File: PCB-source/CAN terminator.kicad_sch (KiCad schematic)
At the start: 6 parts, among them U8 TLP175A, U9 TLP175A

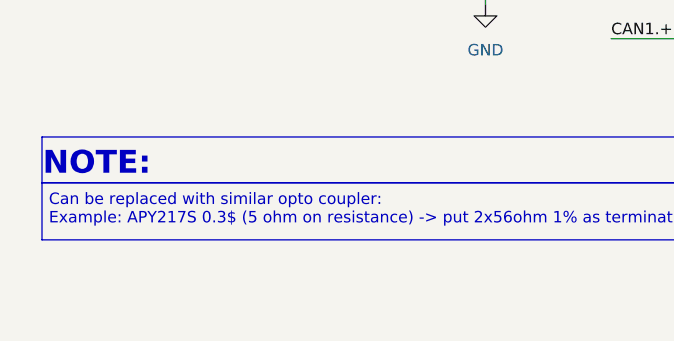
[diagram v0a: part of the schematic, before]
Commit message: bom done
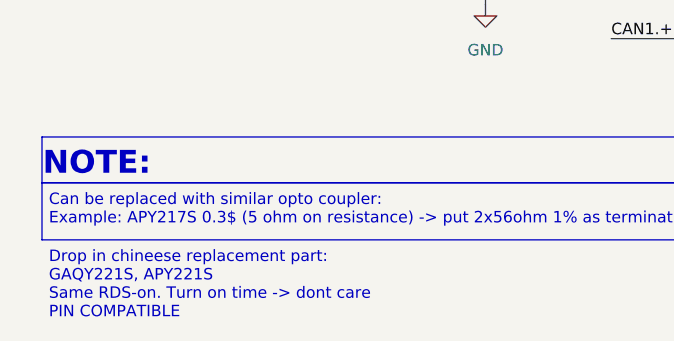
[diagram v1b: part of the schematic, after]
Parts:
- U8, U9: LCSC (none) -> C141522
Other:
- note added: "Drop in chineese replacement part: GAQY221S, APY221S Same RDS-on. Turn on time -> dont care PIN COMPATIBLE"
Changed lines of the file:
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@@
+		)
+	)
+	(text "Drop in chineese replacement part:\nGAQY221S, APY221S\nSame RDS-on. Turn on time -> dont care\nPIN COMPATIBLE"
+		(exclude_from_sim no)
+		(at 44.196 148.082 0)
+		(effects
+			(font
+				(size 1.27 1.27)
+			)
+			(justify left)
 		)
 	)
@@
 		)
 		(property "Description" "MOSFET Photorelay 1-Form-A, Voff 60V, Ion 100mA, SOIC-4-6 (MFSOP-4-6)"
+			(at 110.49 96.52 0)
+			(effects
+				(font
+					(size 1.27 1.27)
+				)
+				(hide yes)
+			)
+		)
+		(property "LCSC" "C141522"
 			(at 110.49 96.52 0)
 			(effects
@@
 			(at 152.4 96.52 0)
 			(effects
+				(font
+					(size 1.27 1.27)
+				)
+				(hide yes)
+			)
+		)
+		(property "LCSC" "C141522"
+			(at 152.4 96.52 0)
+			(effects
